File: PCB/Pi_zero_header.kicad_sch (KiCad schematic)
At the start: 96 parts, among them J1 Raspberry_Pi_2_3, J2 USB_C_Receptacle_USB2.0, J3 Screw_Terminal_01x02, J4 Screw_Terminal_01x02, J5 Conn_02x04_Top_Bottom, J7 Conn_01x04, J8 Conn_02x03_Top_Bottom, J9 Conn_01x02, SW1 SW_Push, SW2 SW_Push, SW3 SW_SPST, U1 RP2040, U2 W25Q128JVS, U3 TB6612FNG, U4 TPS630701RNMR, U5 TPS630701RNMR, U6 PQ25792RQMR, Y1 12M

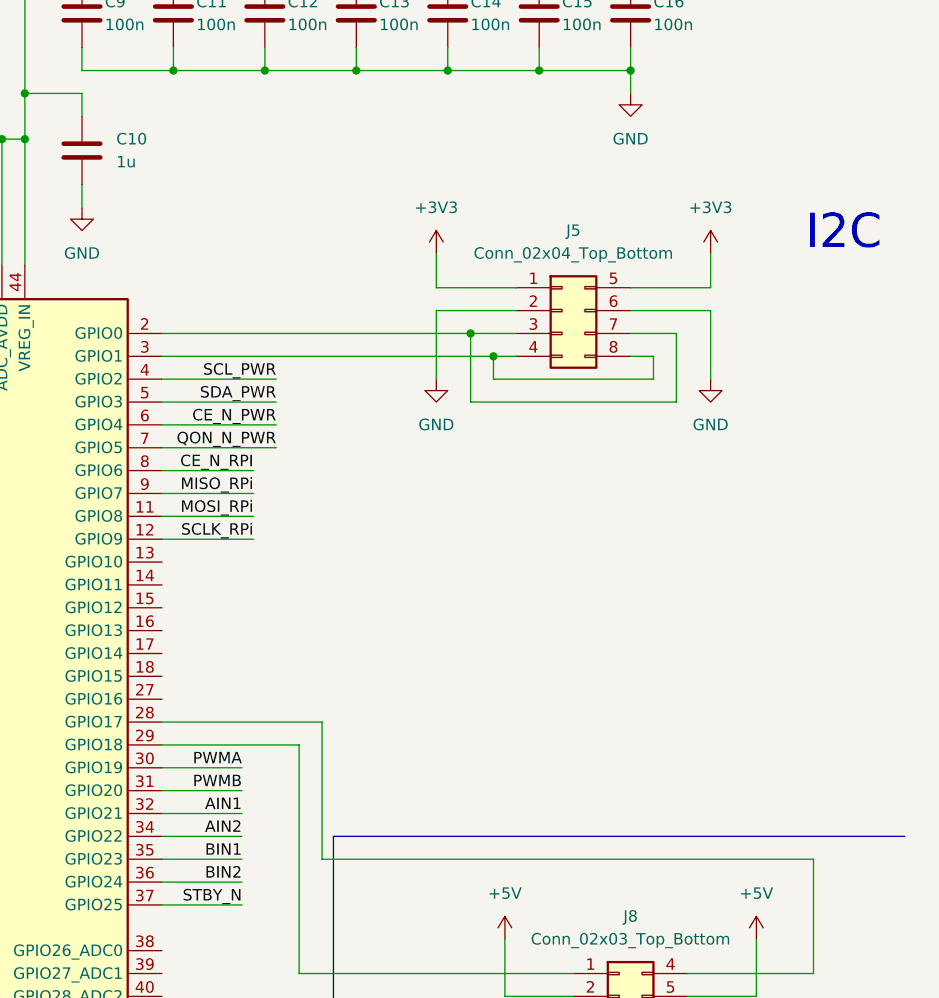
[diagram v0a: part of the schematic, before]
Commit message: I relized I fucked up...
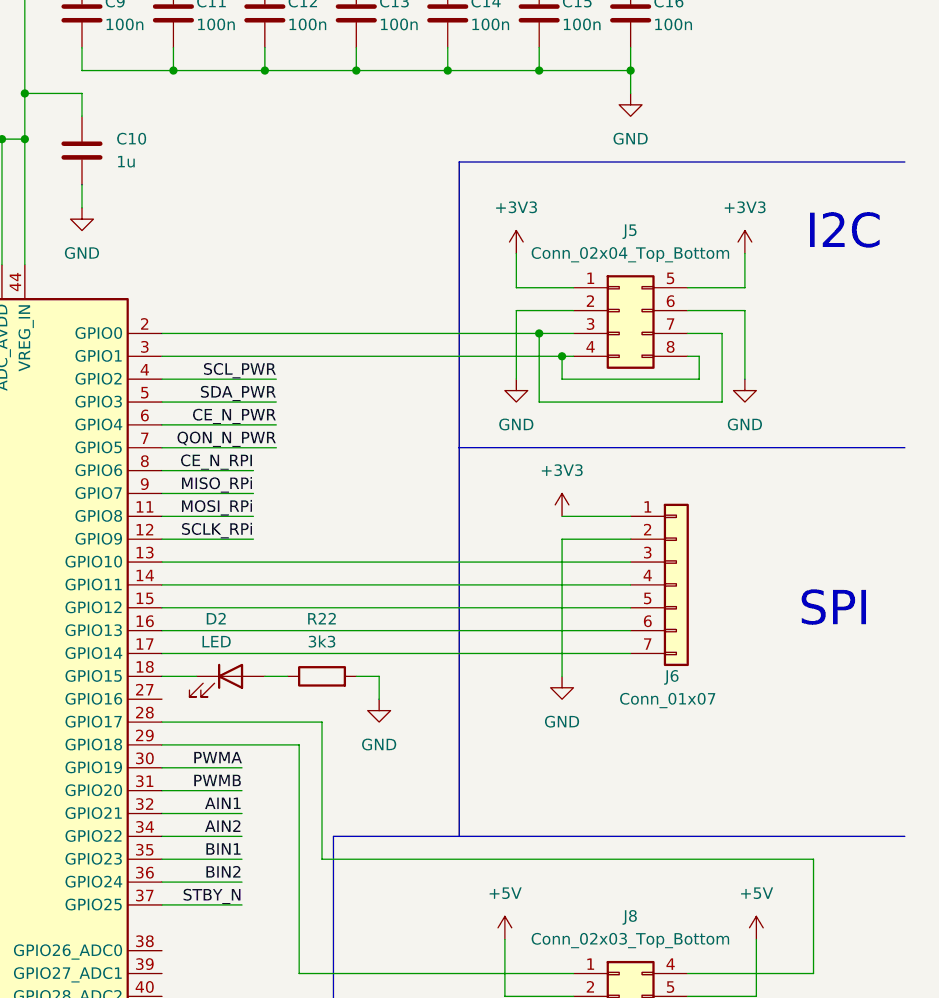
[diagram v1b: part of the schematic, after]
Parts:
- added D2: LED, LED_SMD:LED_0402_1005Metric, symbol Device:LED
- added J6: Conn_01x07, Connector_PinHeader_2.54mm:PinHeader_1x07_P2.54mm_Vertical, symbol Connector_Generic:Conn_01x07
- added R22: 3k3, Resistor_SMD:R_0402_1005Metric, symbol Device:R
- C1, C10, C11, C12, C13, C14, C15, C16, C18, C19, C2, C20, C21, C22, C23, C24, C25, C26, C27, C28, C29, C3, C30, C31, C32, C33, C34, C35, C36, C4, C41, C42, C43, C44, C45, C46, C47, C48, C49, C5, C50, C51, C52, C53, C54, C6, C7, C8, C9: footprint Capacitor_SMD:C_0603_1608Metric -> Capacitor_SMD:C_0402_1005Metric
- D1: footprint LED_SMD:LED_0603_1608Metric -> LED_SMD:LED_0402_1005Metric
- J5: footprint Connector_PinHeader_2.54mm:PinHeader_2x04_P2.54mm_Horizontal -> Connector_PinHeader_2.54mm:PinHeader_2x04_P2.54mm_Vertical
- J7: footprint Connector_PinHeader_2.54mm:PinHeader_1x04_P2.54mm_Horizontal -> Connector_PinHeader_2.54mm:PinHeader_1x04_P2.54mm_Vertical
- J8: footprint Connector_PinHeader_2.54mm:PinHeader_2x03_P2.54mm_Horizontal -> Connector_PinHeader_2.54mm:PinHeader_2x03_P2.54mm_Vertical
- J9: footprint Connector_PinHeader_2.54mm:PinHeader_1x02_P2.54mm_Horizontal -> Connector_PinHeader_2.54mm:PinHeader_1x02_P2.54mm_Vertical
- R1, R10, R11, R12, R13, R14, R15, R16, R17, R18, R19, R2, R20, R21, R3, R4, R5, R6, R7, R8, R9: footprint Resistor_SMD:R_0603_1608Metric -> Resistor_SMD:R_0402_1005Metric
- SW3: footprint Button_Switch_THT:SW_DIP_SPSTx01_Piano_10.8x4.1mm_W7.62mm_P2.54mm -> Button_Switch_THT:SW_CuK_OS102011MA1QN1_SPDT_Angled
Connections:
- net +3V3: now also J6.1 (Pin_1)
- net GND: now also J6.2 (Pin_2), R22.2
- net at U1.13 (GPIO10): now also J6.3 (Pin_3)
- net at U1.14 (GPIO11): now also J6.4 (Pin_4)
- net at U1.15 (GPIO12): now also J6.5 (Pin_5)
- net at U1.16 (GPIO13): now also J6.6 (Pin_6)
- net at U1.17 (GPIO14): now also J6.7 (Pin_7)
- net at U1.18 (GPIO15): now also D2.1 (K)
- new net: D2.2 (A), R22.1
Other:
- note added: "SPI"
- moved on the sheet: J5
